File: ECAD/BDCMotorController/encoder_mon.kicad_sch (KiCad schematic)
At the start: 12 parts, among them U69 74AHC00, U70 74AHC1G17, U71 74AHC1G17, U72 74AHC00, U73 74AHC00

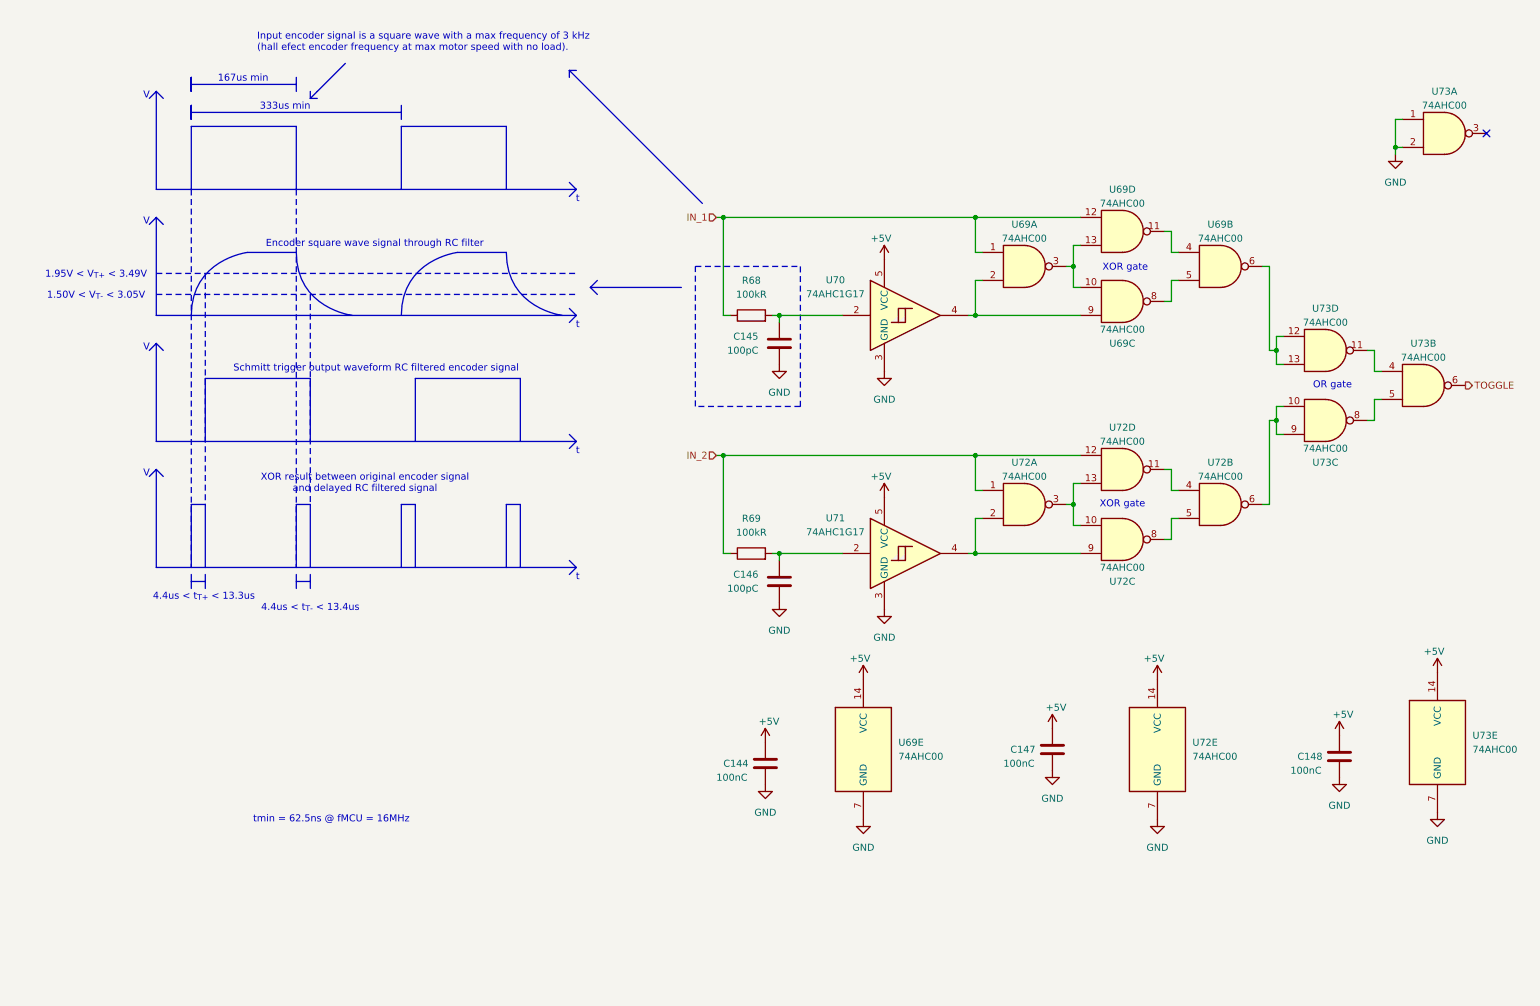
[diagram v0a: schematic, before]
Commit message: Progressed ECAD.
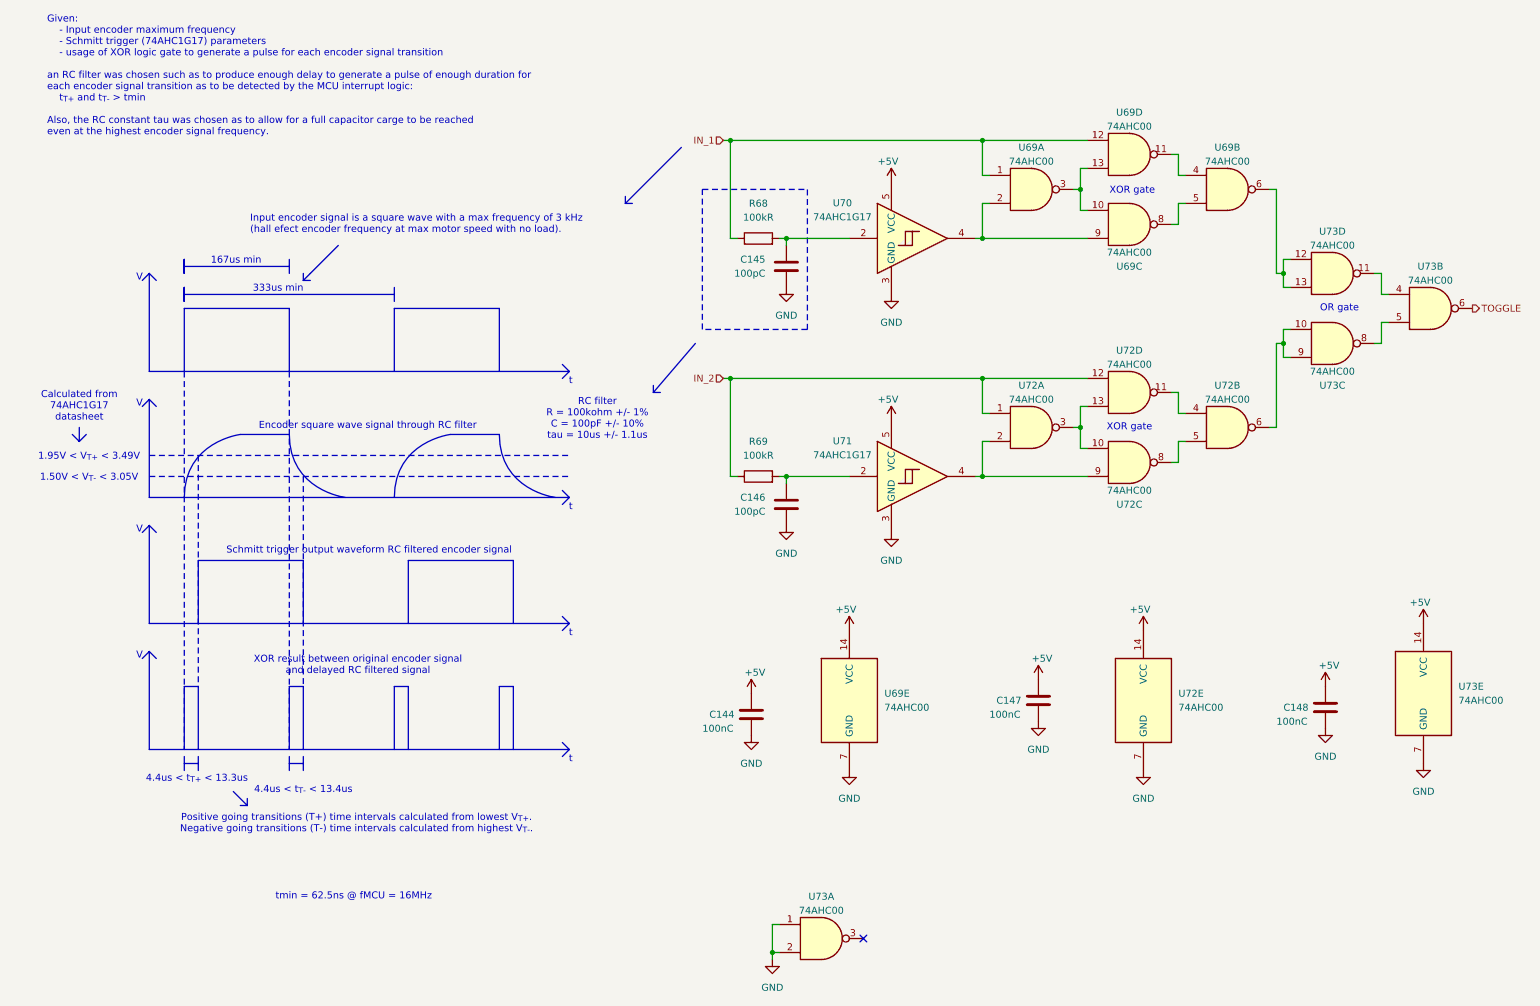
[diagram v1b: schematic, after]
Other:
- note added: "Calculated from 74AHC1G17 datasheet"
- note added: "Given: - Input encoder maximum frequency - Schmitt trigger (74AHC1G17) parameters - usage of XOR logic gate to generate a pulse for each encoder signal transition an RC filter was chosen such as to produce enough delay to generate a pulse of enough duration for each encoder signal transition as to be detected by the MCU interrupt logic: t_{T+} and t_{T-} > tmin Also, the RC constant tau was chose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"
- note added: "Positive going transitions (T+) time intervals calculated from lowest V_{T+}. Negative going transitions (T-) time intervals calculated from highest V_{T-}."
- note added: "RC filter R = 100kohm +/- 1% C = 100pF +/- 10% tau = 10us +/- 1.1us"
- moved on the sheet: C144, C145, C146, C147, C148, R68, R69, U69A, U69B, U69C, U69D, U69E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
